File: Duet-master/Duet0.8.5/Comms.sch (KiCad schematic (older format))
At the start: 42 parts, among them J19 USB, J20 uSDHC, J21 ETHERNET, U11 KSZ8051RNL, X1 CRYSTAL_4PIN

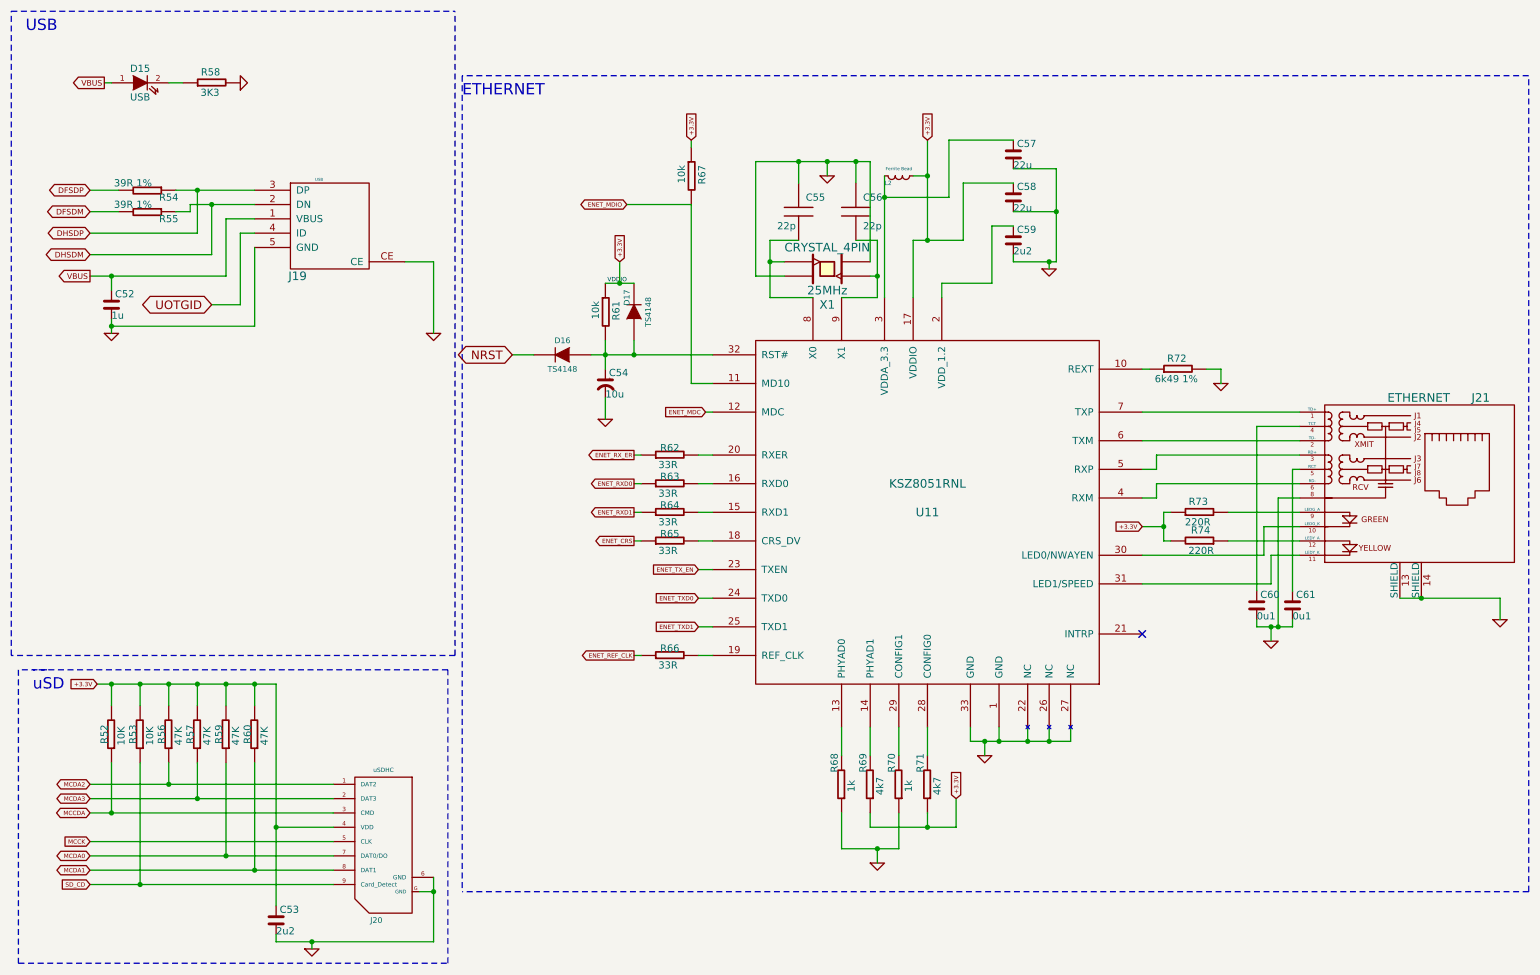
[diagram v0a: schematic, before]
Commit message: PCB layout of components started
Experienced advice welcome.
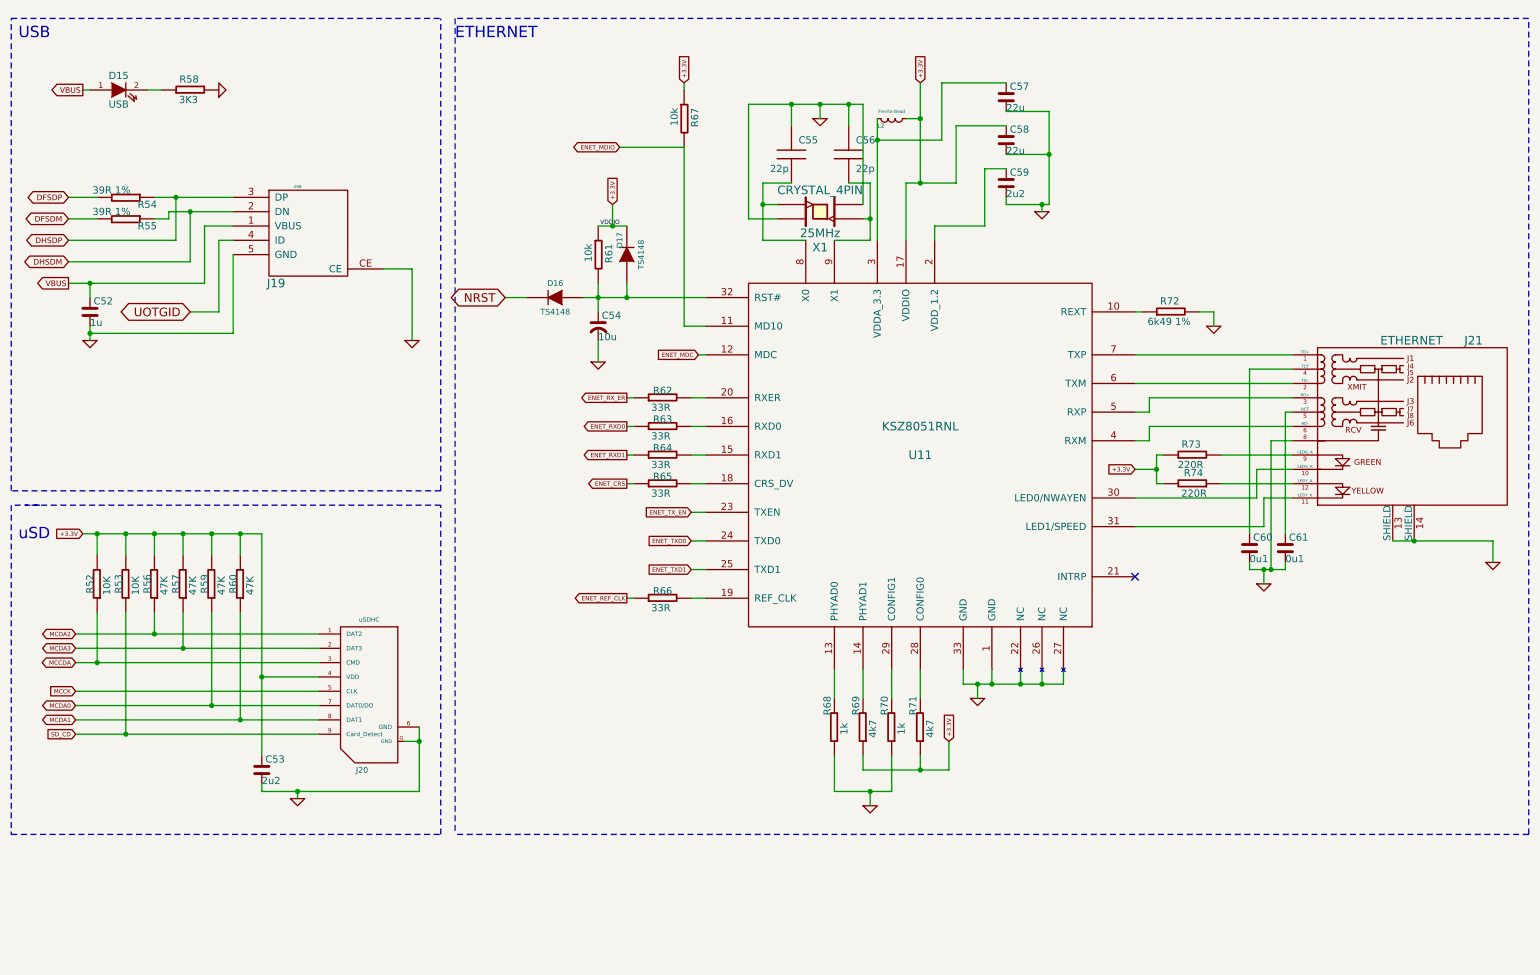
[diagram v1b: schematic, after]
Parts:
- C52: footprint (none) -> Melter_Connections:1mf_capacitor
- C53, C59: footprint (none) -> Melter_Connections:2mf2_capacitor
- C54: footprint (none) -> Melter_Connections:10mf_capacitor
- C55, C56: footprint (none) -> Melter_Connections:22pf_capacitor
- C57, C58: footprint (none) -> Melter_Connections:22mf_Capacitor_1210
- C60, C61: footprint (none) -> Melter_Connections:0mf1_capacitor
- D15: footprint (none) -> Melter_Connections:USB_Diode_0603
- D16, D17: footprint (none) -> Melter_Connections:TS4148_Diode_0805
- J19: footprint (none) -> Melter_Connections:USB_B
- J20: footprint (none) -> Melter_Connections:SD_Card_Receptacle
- J21: footprint (none) -> Melter_Connections:RJ45_MAG
- L2: footprint 1206 -> Melter_Connections:FERRITE_BEAD
- R52, R53, R61, R67: footprint 0603 -> Melter_Connections:10k_R_0603
- R54, R55: footprint (none) -> Melter_Connections:39_1per_R_0603
- R56, R57, R59, R60: footprint 0603 -> Melter_Connections:47k_R_0603
- R58: footprint (none) -> Melter_Connections:3k3_R_0603
- R62, R63, R64, R65, R66: footprint 0603 -> Melter_Connections:33R_R_0603
- R68, R70: footprint 0603 -> Melter_Connections:1k_R_0603
- R69, R71: footprint 0603 -> Melter_Connections:4k7_R_0603
- R72: footprint 0603 -> Melter_Connections:6k49_1_per_R_0603
- R73, R74: footprint 0603 -> Melter_Connections:220R_R_0603
- U11: footprint (none) -> Melter_Connections:KSZ8051RNL
- X1: footprint (none) -> Melter_Connections:Xtal_5x3.2
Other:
- moved on the sheet: C52, C53, C54, C55, C56, C57, C58, C59, C60, C61, D15, D16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

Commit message: USB 3 receptacles!
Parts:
- J19: footprint Melter_Connections:USB_B -> Melter_Connections:uSD_SKT
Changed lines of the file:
@@
 Connection ~ 6400 1150
 Wire Wire Line
-	6500 1150 6400 1150
-Wire Wire Line
-	6400 1150 6200 1150
-Wire Wire Line
-	6200 1150 6000 1150
-Wire Wire Line
-	6000 1150 5700 1150
+	5700 1150 6500 1150
 Wire Wire Line
 	6500 1150 6500 1850
 Connection ~ 5800 1850
 Wire Wire Line
-	5800 2100 5800 1850
-Wire Wire Line
-	5800 1850 5800 1700
+	5800 1700 5800 2100
 Wire Wire Line
 	5800 2100 6100 2100
@@
 	2000 2600 1800 2600
 Wire Wire Line
-	1100 2800 1100 2750
-Wire Wire Line
-	1100 2750 1100 2700
+	1100 2700 1100 2800
 Wire Wire Line
 	5250 1050 5250 1000
 Connection ~ 2300 5150
 Wire Wire Line
-	1000 5450 2150 5450
-Wire Wire Line
-	2150 5450 2700 5450
+	1000 5450 2700 5450
 Wire Wire Line
 	1000 5250 2700 5250
 Wire Wire Line
-	1000 4950 1750 4950
-Wire Wire Line
-	1750 4950 2700 4950
+	1000 4950 2700 4950
 Connection ~ 3400 5600
 Wire Wire Line
-	3400 5500 3400 5600
-Wire Wire Line
-	3400 5600 3400 5950
-Wire Wire Line
-	3400 5950 2550 5950
-Wire Wire Line
-	2550 5950 2300 5950
+	3400 5950 3400 5500
+Wire Wire Line
+	2300 5950 3400 5950
 Wire Notes Line
 	3550 3850 550  3850
@@
 	9500 3100 8400 3100
 Wire Wire Line
-	8600 3800 8550 3800
-Wire Wire Line
-	8550 3800 8550 3700
-Wire Wire Line
-	8550 3700 8550 3600
+	8550 3800 8600 3800
+Wire Wire Line
+	8550 3600 8550 3800
 Wire Wire Line
 	8550 3600 8600 3600
@@
 	3650 550  3650 6250
 Wire Wire Line
-	1900 2400 1100 2400
-Wire Wire Line
-	1100 2400 950  2400
+	1900 2400 950  2400
 Wire Wire Line
 	950  1800 1150 1800
 Connection ~ 6900 5800
 Wire Wire Line
-	7100 5600 7100 5800
-Wire Wire Line
-	7100 5800 6900 5800
-Wire Wire Line
-	6900 5800 6500 5800
+	7100 5800 7100 5600
+Wire Wire Line
+	6500 5800 7100 5800
 Wire Wire Line
 	6500 5800 6500 5700
@@
 Connection ~ 4850 2500
 Wire Wire Line
-	5400 2500 4850 2500
-Wire Wire Line
-	4850 2500 4650 2500
-Wire Wire Line
-	4650 2500 4550 2500
+	4550 2500 5400 2500
 Wire Wire Line
 	4650 2950 4650 2800
 Connection ~ 6900 1250
 Wire Wire Line
-	6900 1000 6900 1250
-Wire Wire Line
-	6900 1250 6900 1700
+	6900 1000 6900 1700
 Wire Wire Line
 	6800 1250 6900 1250
@@
 Connection ~ 7750 5200
 Wire Wire Line
-	7900 5100 7900 5200
-Wire Wire Line
-	7900 5200 7750 5200
-Wire Wire Line
-	7750 5200 7600 5200
-Wire Wire Line
-	7600 5200 7400 5200
-Wire Wire Line
-	7400 5200 7300 5200
-Wire Wire Line
-	7300 5200 7200 5200
+	7900 5200 7900 5100
+Wire Wire Line
+	7200 5200 7900 5200
 Connection ~ 7400 5200
 Wire Wire Line
@@
 Connection ~ 7800 1500
 Wire Wire Line
-	6600 1250 6600 1400
-Wire Wire Line
-	6600 1400 6600 2100
+	6600 1250 6600 2100
 Connection ~ 6600 1400
 Connection ~ 6900 1700
@@
 Connection ~ 4650 2500
 Wire Wire Line
-	4650 2600 4650 2500
-Wire Wire Line
-	4650 2500 4650 2400
-Wire Wire Line
-	4850 2000 4750 2000
-Wire Wire Line
-	4750 2000 4650 2000
+	4650 2400 4650 2600
+Wire Wire Line
+	4650 2000 4850 2000
 Wire Wire Line
 	5300 3600 5400 3600
@@
 	950  1950 1150 1950
 Wire Wire Line
-	1550 1800 1700 1800
-Wire Wire Line
-	1700 1800 2100 1800
-Wire Wire Line
-	2100 1900 1800 1900
-Wire Wire Line
-	1800 1900 1650 1900
+	1550 1800 2100 1800
+Wire Wire Line
+	1650 1900 2100 1900
 Wire Wire Line
 	1650 1900 1650 1950
@@
 	9500 3800 9000 3800
 Wire Wire Line
-	9450 4350 9450 4400
-Wire Wire Line
-	9450 4400 9350 4400
-Wire Wire Line
-	9350 4400 9300 4400
-Wire Wire Line
-	9300 4400 9200 4400
+	9450 4400 9450 4350
+Wire Wire Line
+	9200 4400 9450 4400
 Wire Wire Line
 	9200 4400 9200 4350
@@
 	2700 5150 2300 5150
 Wire Wire Line
-	2300 5700 2300 5150
-Wire Wire Line
-	2300 5150 2300 4150
-Wire Wire Line
-	1000 4850 1550 4850
-Wire Wire Line
-	1550 4850 2700 4850
-Wire Wire Line
-	1000 5050 1150 5050
-Wire Wire Line
-	1150 5050 2700 5050
-Wire Wire Line
-	1000 5350 1950 5350
-Wire Wire Line
-	1950 5350 2700 5350
-Wire Wire Line
-	1000 5550 1350 5550
-Wire Wire Line
-	1350 5550 2700 5550
+	2300 4150 2300 5700
+Wire Wire Line
+	1000 4850 2700 4850
+Wire Wire Line
+	1000 5050 2700 5050
+Wire Wire Line
+	1000 5350 2700 5350
+Wire Wire Line
+	1000 5550 2700 5550
 Wire Wire Line
 	5400 2700 5250 2700
@@
 	5800 1700 6000 1700
 Wire Wire Line
-	6300 2100 6550 2100
-Wire Wire Line
-	6550 2100 6550 1950
-Wire Wire Line
-	6550 1950 6550 1700
+	6550 2100 6300 2100
+Wire Wire Line
+	6550 1700 6550 2100
 Connection ~ 6550 1950
 Wire Wire Line
@@
 	6300 5700 6300 5950
 Wire Wire Line
-	6300 5950 6550 5950
-Wire Wire Line
-	6550 5950 6700 5950
+	6300 5950 6700 5950
 Wire Wire Line
 	6700 5950 6700 5700
 Wire Wire Line
-	2300 4150 2150 4150
-Wire Wire Line
-	2150 4150 1950 4150
-Wire Wire Line
-	1950 4150 1750 4150
-Wire Wire Line
-	1750 4150 1550 4150
-Wire Wire Line
-	1550 4150 1350 4150
-Wire Wire Line
-	1350 4150 1150 4150
-Wire Wire Line
-	1150 4150 1050 4150
+	1050 4150 2300 4150
 Wire Wire Line
 	1950 4700 1950 5350
@@
 Connection ~ 1150 4150
 Wire Wire Line
-	7800 1200 7800 1500
-Wire Wire Line
-	7800 1500 7800 1850
-Wire Wire Line
-	7800 1850 7750 1850
-Wire Wire Line
-	7750 1850 7500 1850
+	7800 1200 7800 1850
+Wire Wire Line
+	7800 1850 7500 1850
 Connection ~ 7750 1850
 Wire Wire Line
@@
 	2100 2750 2100 2200
 Wire Wire Line
-	10200 4200 10350 4200
-Wire Wire Line
-	10350 4200 10900 4200
+	10200 4200 10900 4200
 Connection ~ 10350 4200
 Wire Wire Line
-	6800 1700 6900 1700
-Wire Wire Line
-	6900 1700 7150 1700
+	6800 1700 7150 1700
 Wire Wire Line
 	7150 1700 7150 1300
@@
 F 0 "J19" H 2400 1700 60  0000 C CNN
 F 1 "USB" H 2550 2375 20  0000 C CNN
-F 2 "Melter_Connections:USB_B" H 2700 2050 60  0001 C CNN
+F 2 "Melter_Connections:uSD_SKT" H 2700 2050 60  0001 C CNN
 F 3 "" H 2700 2050 60  0001 C CNN
 	1    2700 2050
